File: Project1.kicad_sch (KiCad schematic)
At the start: 65 parts, among them IC1 LM324N, IC2 LM324N, IC3 LM324N, U3 LM324

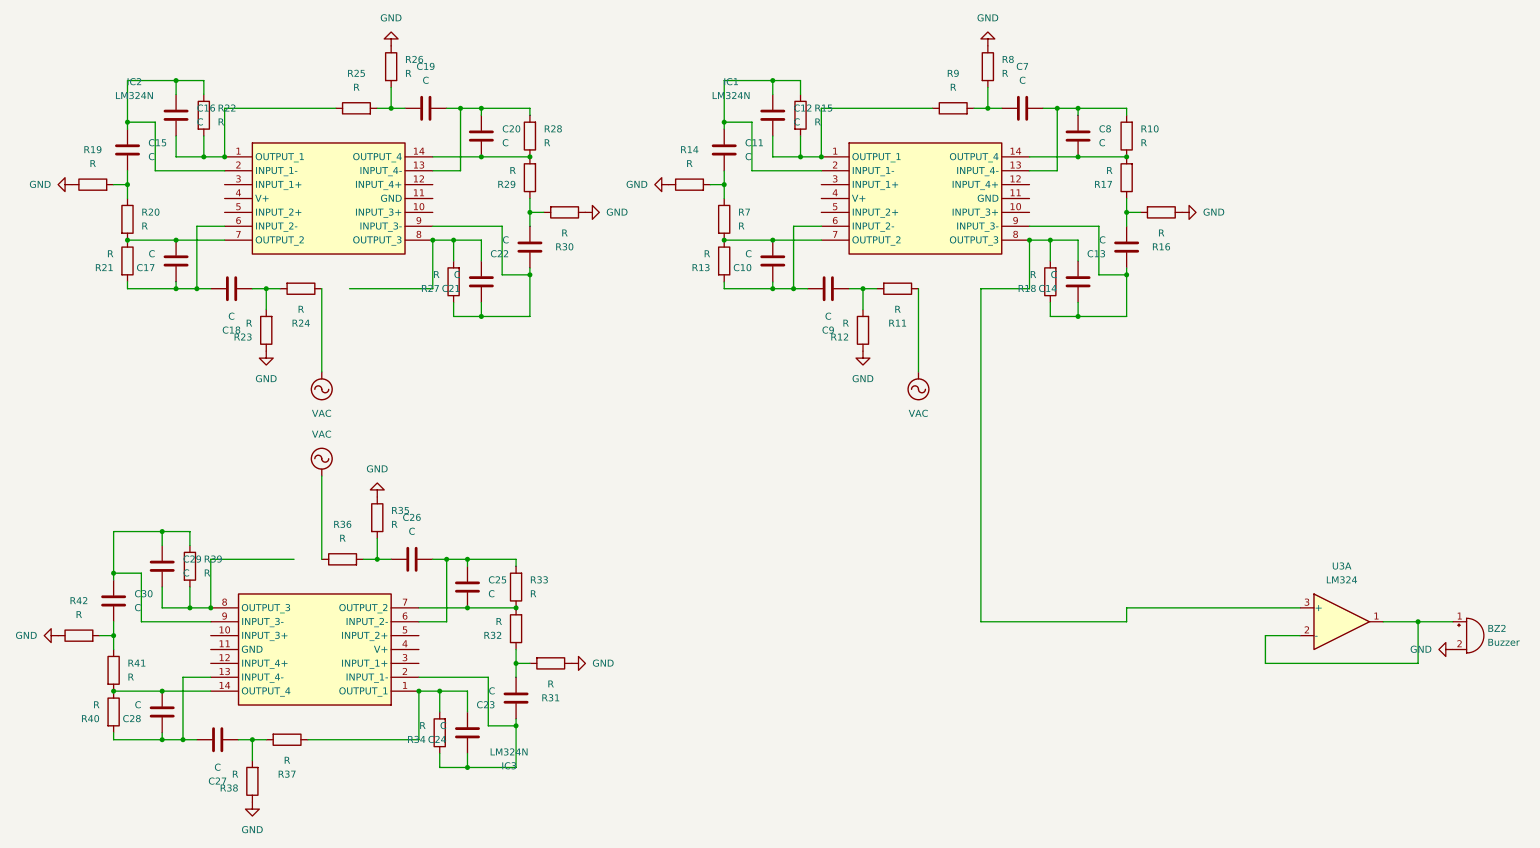
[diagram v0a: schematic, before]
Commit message: dd
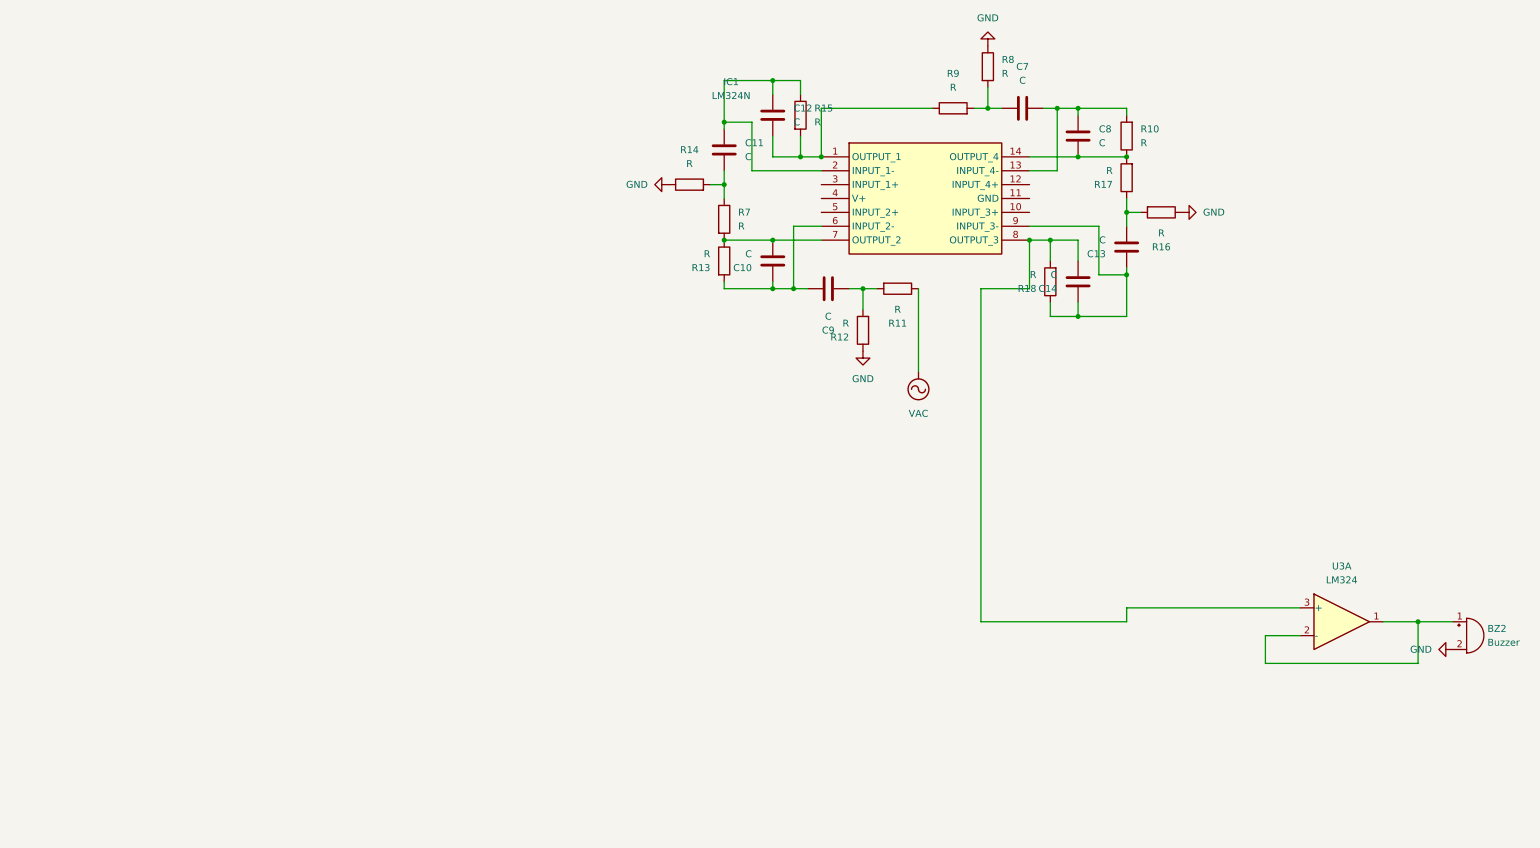
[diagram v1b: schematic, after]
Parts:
- removed C15, C16, C17, C18, C19, C20, C21, C22, C23, C24, C25, C26, C27, C28, C29, C30: C, symbol Device:C
- removed IC2, IC3: LM324N, DIP794W56P254L1905H533Q14N, symbol New_Library:LM324N
- removed R19, R20, R21, R22, R23, R24, R25, R26, R27, R28, R29, R30, R31, R32, R33, R34, R35, R36, R37, R38, R39, R40, R41, R42: R, symbol Device:R

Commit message: 0518_11:23 edited.
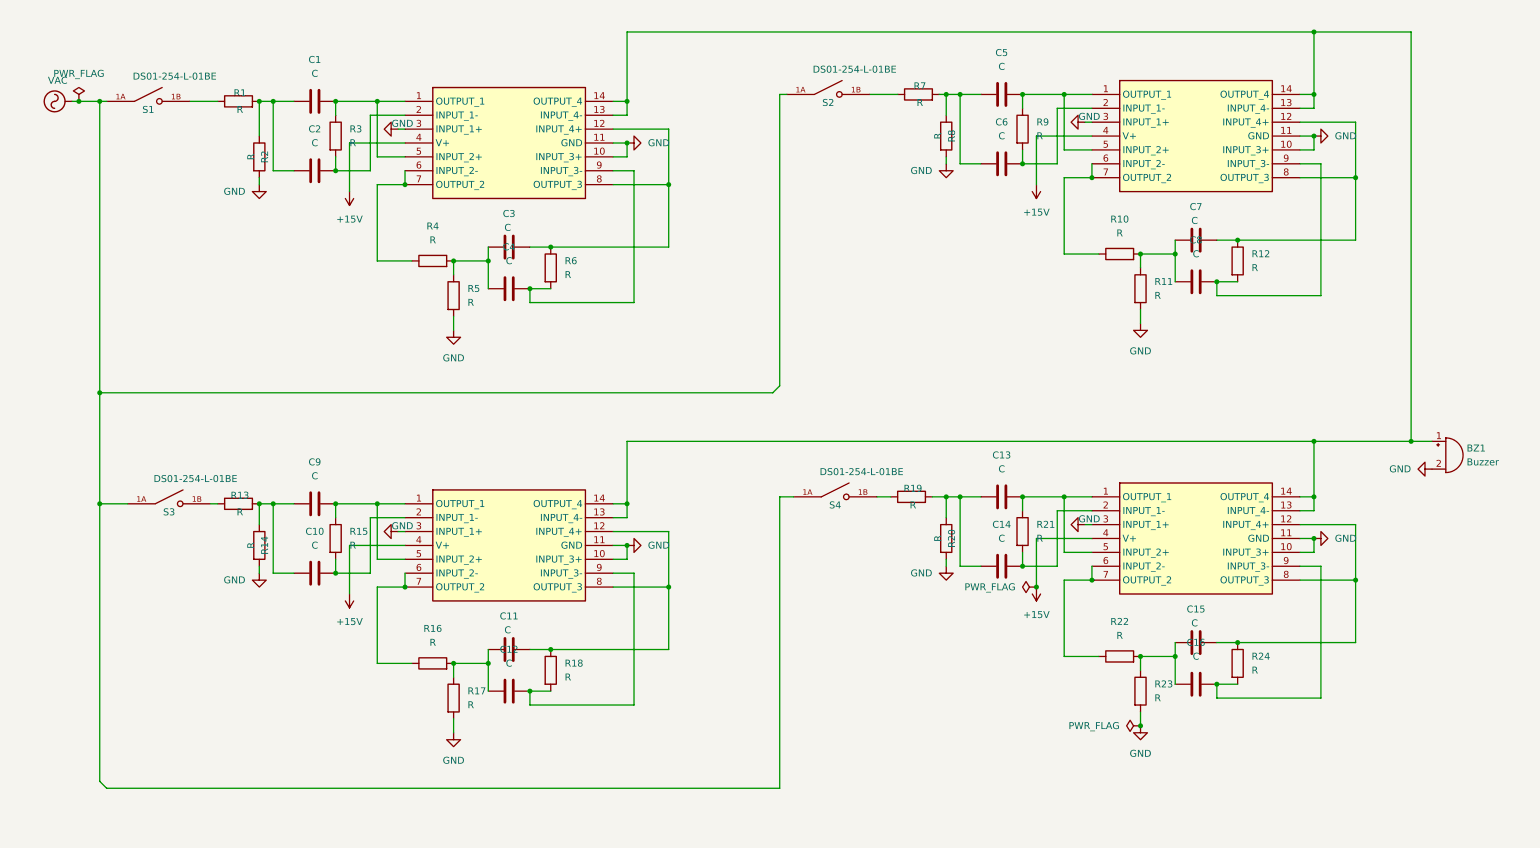
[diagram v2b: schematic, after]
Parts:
- removed BZ2: Buzzer, symbol Device:Buzzer
- removed U3: LM324, symbol Amplifier_Operational:LM324
- added BZ1: Buzzer, Buzzer_Beeper:Buzzer_12x9.5RM7.6, symbol Device:Buzzer
- added C1, C15, C16, C2, C3, C4, C5, C6: C, Capacitor_SMD:C_0603_1608Metric, symbol Device:C
- added IC2, IC3, IC4: LM324N, Project1:LM324N, symbol New_Library:LM324N
- added R1, R19, R2, R20, R21, R22, R23, R24, R3, R4, R5, R6: R, Resistor_SMD:R_0603_1608Metric, symbol Device:R
- added S1, S2, S3, S4: DS01-254-L-01BE, Project1:SW_DS01-254-L-01BE, symbol New_Library:DS01-254-L-01BE
- C10, C11, C12, C13, C14, C7, C8, C9: footprint (none) -> Capacitor_SMD:C_0603_1608Metric
- IC1: footprint DIP794W56P254L1905H533Q14N -> Project1:LM324N
- R10, R11, R12, R13, R14, R15, R16, R17, R18, R7, R8, R9: footprint (none) -> Resistor_SMD:R_0603_1608Metric
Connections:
- net GND: now also IC1.10 (INPUT_3+), IC1.11 (GND), IC1.3 (INPUT_1+), R11.2, R14.2, R17.2, R8.2, BZ1.2 (-), IC2.10 (INPUT_3+), IC2.11 (GND), IC2.3 (INPUT_1+), IC3.10 (INPUT_3+), IC3.11 (GND), IC3.3 (INPUT_1+), IC4.10 (INPUT_3+), IC4.11 (GND), IC4.3 (INPUT_1+), R2.2, R20.2, R23.2, R5.2; no longer R12.1, R14.1, R16.1, R8.1
- net VAC: now also S1.1A, S2.1A, S3.1A, S4.1A; no longer R11.1
- net at IC1.12 (INPUT_4+): now also IC1.8 (OUTPUT_3), C3.2, R6.1
- net at C8.1, R10.2: now also C7.1, R11.1; no longer C7.2, IC1.13 (INPUT_4-)
- net at C11.1, C12.1: now also R16.2, R17.1; no longer IC1.2 (INPUT_1-), R15.1
- net +15V: now reaches IC1.4 (V+)
- net +15V: now also IC2.4 (V+), IC3.4 (V+), IC4.4 (V+)
- net at IC1.5 (INPUT_2+): now also IC1.1 (OUTPUT_1), C1.1, R3.1
- net at C10.1, C9.2, R13.2: now also R14.1; no longer IC1.6 (INPUT_2-)
- new net: C1.2, C2.1, R1.2, R2.1
- new net: C13.2, C14.1, R19.2, R20.1
- new net: C14.2, IC4.2 (INPUT_1-), R21.2
- new net: C3.1, C4.1, R4.2, R5.1
- new net: R7.1, S2.1B
- new net: C5.2, C6.1, R7.2, R8.1
- new net: BZ1.1 (+), IC1.13 (INPUT_4-), IC1.14 (OUTPUT_4), IC2.13 (INPUT_4-), IC2.14 (OUTPUT_4), IC3.13 (INPUT_4-), IC3.14 (OUTPUT_4), IC4.13 (INPUT_4-), IC4.14 (OUTPUT_4)
- new net: C11.2, IC3.12 (INPUT_4+), IC3.8 (OUTPUT_3), R18.1
- new net: C4.2, IC1.9 (INPUT_3-), R6.2
- new net: C15.1, C16.1, R22.2, R23.1
- new net: C9.1, IC3.1 (OUTPUT_1), IC3.5 (INPUT_2+), R15.1
- new net: C10.2, IC3.2 (INPUT_1-), R15.2
- new net: IC3.6 (INPUT_2-), IC3.7 (OUTPUT_2), R16.1
- new net: C12.2, IC3.9 (INPUT_3-), R18.2
- new net: R19.1, S4.1B
- new net: C5.1, IC2.1 (OUTPUT_1), IC2.5 (INPUT_2+), R9.1
- new net: R13.1, S3.1B
- new net: IC2.6 (INPUT_2-), IC2.7 (OUTPUT_2), R10.1
- new net: C16.2, IC4.9 (INPUT_3-), R24.2
- new net: C15.2, IC4.12 (INPUT_4+), IC4.8 (OUTPUT_3), R24.1
- new net: C7.2, IC2.12 (INPUT_4+), IC2.8 (OUTPUT_3), R12.1
- new net: C6.2, IC2.2 (INPUT_1-), R9.2
- new net: C13.1, IC4.1 (OUTPUT_1), IC4.5 (INPUT_2+), R21.1
- new net: C8.2, IC2.9 (INPUT_3-), R12.2
- new net: IC4.6 (INPUT_2-), IC4.7 (OUTPUT_2), R22.1
- new net: R1.1, S1.1B
- new net: C2.2, IC1.2 (INPUT_1-), R3.2
- new net: IC1.6 (INPUT_2-), IC1.7 (OUTPUT_2), R4.1
